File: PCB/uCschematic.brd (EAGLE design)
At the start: 82.5 x 75.5 mm, 63 parts, among them IC1 PIC24FJXXGA002/SO, IC10 ULN2003D1013TR, IC11 ULN2003D1013TR, IC12 ULN2003D1013TR, IC13 FT230XS-U, IC2 317EMP, IC3 MC74HC175ADG, IC4 MC74HC175ADG, IC5 MC74HC175ADG, IC6 MC74HC175ADG, IC7 MC74HC175ADG, IC8 MC74HC175ADG, IC9 ULN2003D1013TR, J1 UJ2-BH-1-TH, J8 68000-105HTLF, J9 68000-105HTLF, U1 74HC237D-Q100J

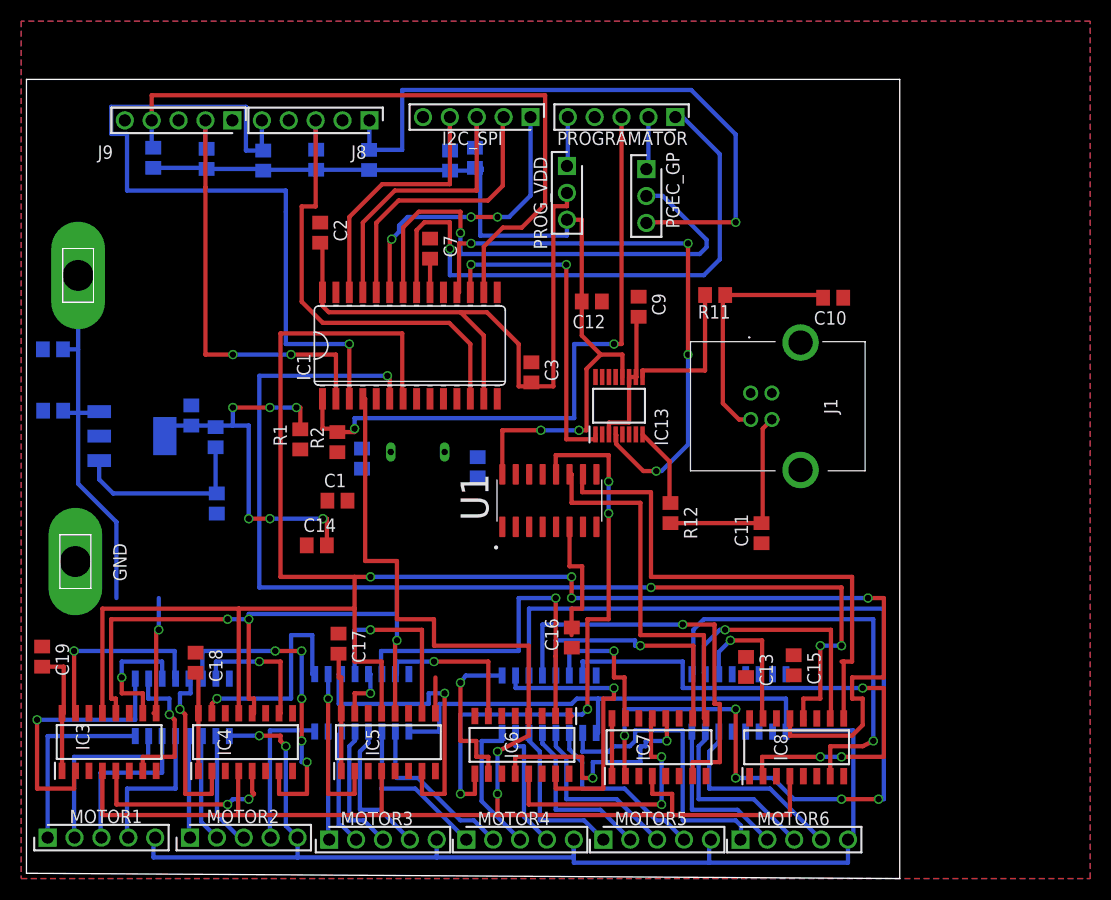
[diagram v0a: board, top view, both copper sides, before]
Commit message: Valjda gotovo
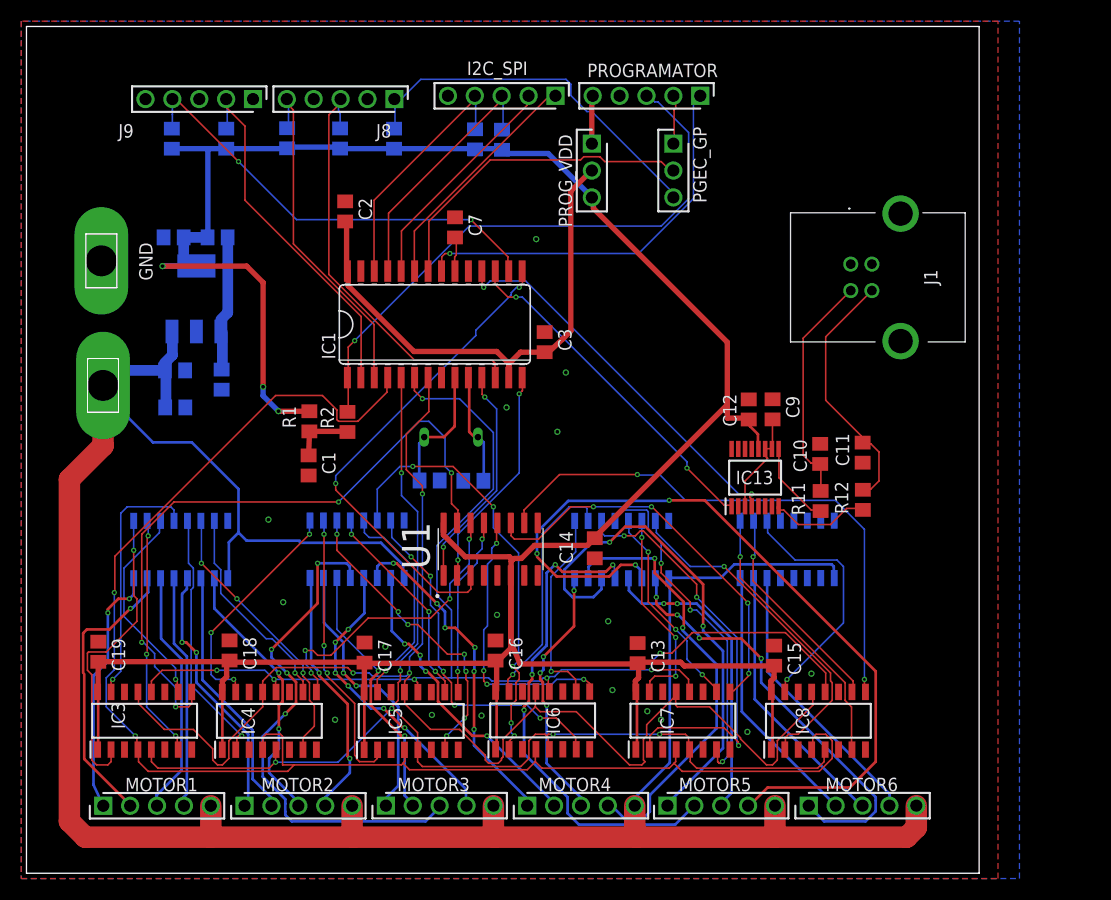
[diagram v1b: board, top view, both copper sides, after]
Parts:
- moved GND 28.5 mm to (7.08, 57.9)
- moved C14 26.3 mm to (53.7, 30.7), turned to 90 degrees
- moved R11 21.9 mm to (75.0, 35.2), turned to 90 degrees
- moved R3 18.9 mm to (18.1, 60.1), turned to 0 degrees
- moved R12 18.2 mm to (79.0, 35.3), turned to 90 degrees
- moved C12 18.0 mm to (68.2, 43.8), turned to 270 degrees
- moved C4 16.9 mm to (13.9, 60.1), turned to 180 degrees
- moved IC11 16.1 mm to (56.2, 30.6)
- moved C9 15.9 mm to (70.5, 43.8)
- moved J1 15.4 mm to (88.7, 56.3)
- moved IC12 15.2 mm to (71.9, 30.6)
- moved IC9 14.9 mm to (14.6, 30.6)
- moved C10 14.8 mm to (75.0, 39.6), turned to 270 degrees
- moved IC13 14.5 mm to (68.8, 37.4)
- moved IC10 14.5 mm to (31.2, 30.6)
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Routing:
- net 3.3V: track 177.7 -> 284.2 mm, vias 8 -> 3
- net N$18: track 18.8 -> 113.0 mm, vias 2 -> 6
- net N$12: track 208.4 -> 130.9 mm, vias 6 -> 3
- net N$13: track 187.8 -> 116.8 mm, vias 9 -> 7
- net N$67: track 17.4 -> 76.8 mm, vias 0 -> 3
- net M4_0: track 96.1 -> 40.3 mm, vias 5 -> 3
- net M0: track 11.2 -> 62.8 mm, vias 1 -> 4
- net N$16: track 0.00 -> 46.3 mm, vias 0 -> 2
- net 12V: track 194.2 -> 239.3 mm, vias 2 -> 0
- net N$29: track 71.5 -> 32.6 mm, vias 1 -> 0
- net N$49: track 12.5 -> 48.6 mm, vias 0 -> 4
- net N$64: track 15.4 -> 47.9 mm, vias 0 -> 2
- net N$65: track 16.0 -> 46.9 mm, vias 0 -> 4
- net N$63: track 11.8 -> 41.5 mm, vias 0 -> 2
- net M3: track 55.8 -> 26.7 mm
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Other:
- board size 82.5 x 75.5 mm -> 90 x 80 mm
